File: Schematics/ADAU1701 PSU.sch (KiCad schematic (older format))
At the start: 56 parts, among them P301 PIN, P302 PIN, P303 PIN, P304 CONN_2x1, P305 CONN_2x1, P306 PIN, U301 IC-REG-XRP7659ISTR-F, U302 NCP700BSN33T1G, U303 NCP700BSN33T1G, U304 NCP700BSN18T1G

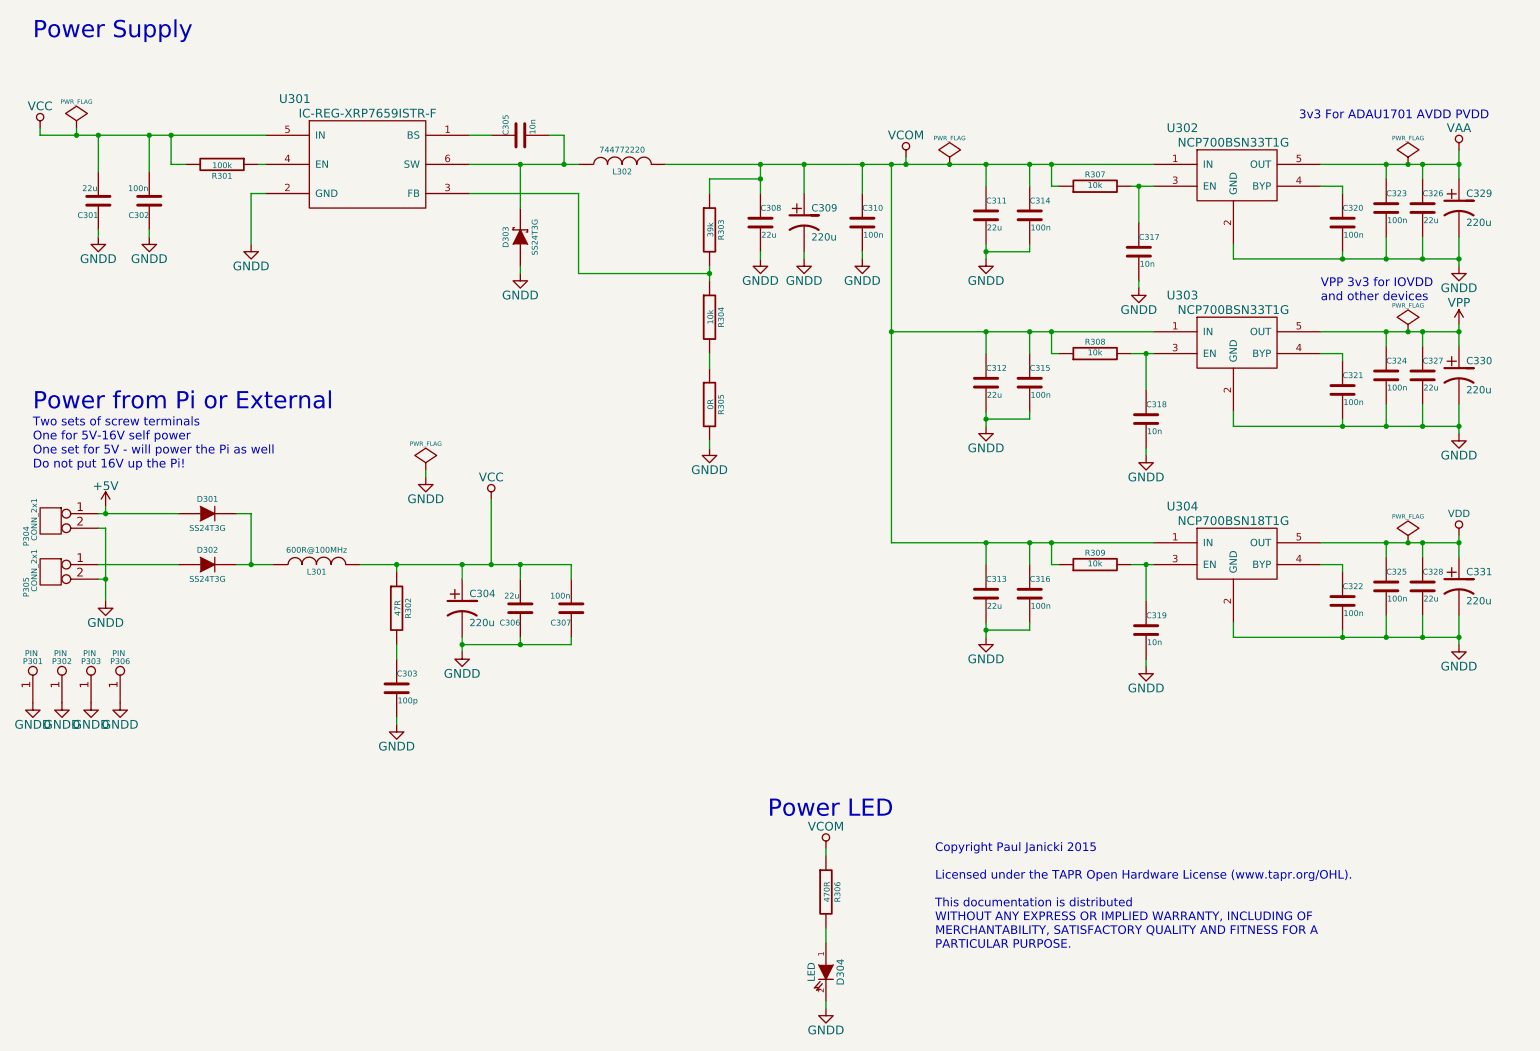
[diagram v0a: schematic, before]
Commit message: WIP PSU changes
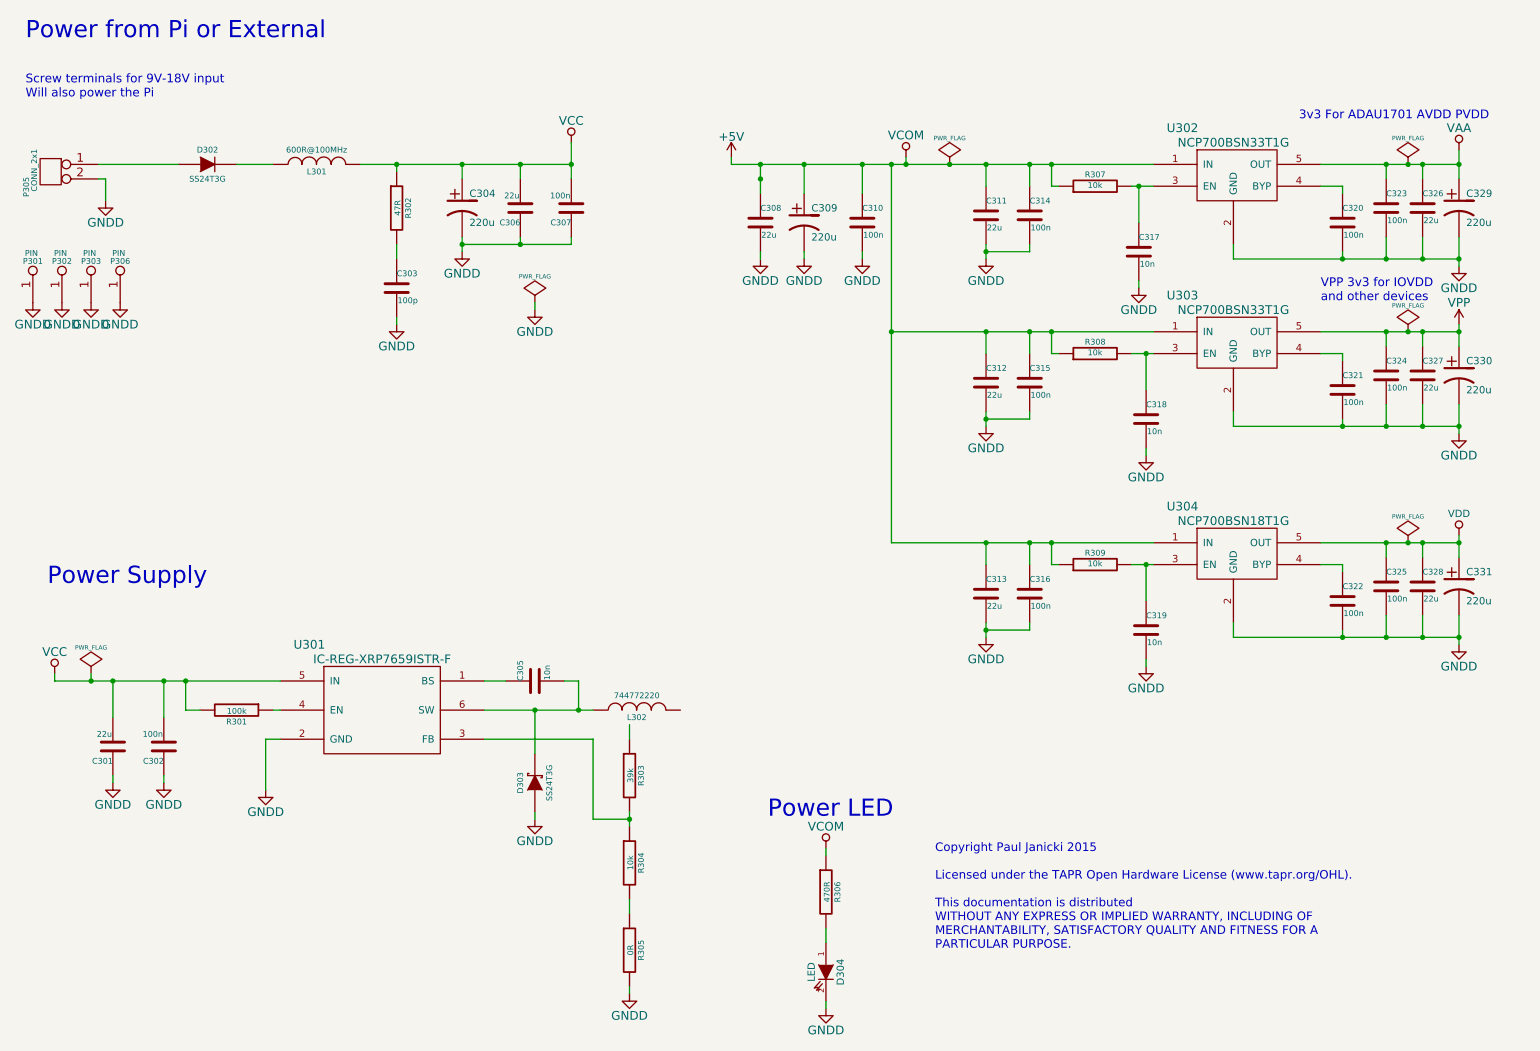
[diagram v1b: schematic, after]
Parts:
- removed D301: SS24T3G, OHDSP-Footprints-Pretty:DIODE-SMB, symbol DIODE
- removed P304: CONN_2x1, OHDSP-Footprints-Pretty:CONN_SIL_2, symbol CONN_2x1
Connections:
- net +5V: now also C308.1, C309.1, C310.1, C311.1, C312.1, C313.1, C314.1, C315.1, C316.1, R306.1, R307.1, R308.1, R309.1, U302.1 (IN), U303.1 (IN), U304.1 (IN)
- removed net VCOM: C308.1, C309.1, C310.1, C311.1, C312.1, C313.1, C314.1, C315.1, C316.1, L302.2, R303.1, R306.1, R307.1, R308.1, R309.1, U302.1 (IN), U303.1 (IN), U304.1 (IN)
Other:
- note added: "Screw terminals for 9V-18V input\nWill also power the Pi"
- note removed: "Two sets of screw terminals\nOne for 5V-16V self power\nOne set for 5V - will power the Pi as well\nDo not put 16V up the Pi!"
- moved on the sheet: C301, C302, C303, C304, C305, C306, C307, D302, D303, L301, L302, P301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
